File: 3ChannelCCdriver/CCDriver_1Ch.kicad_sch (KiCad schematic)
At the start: 7 parts, among them U1 AL8860WT-7

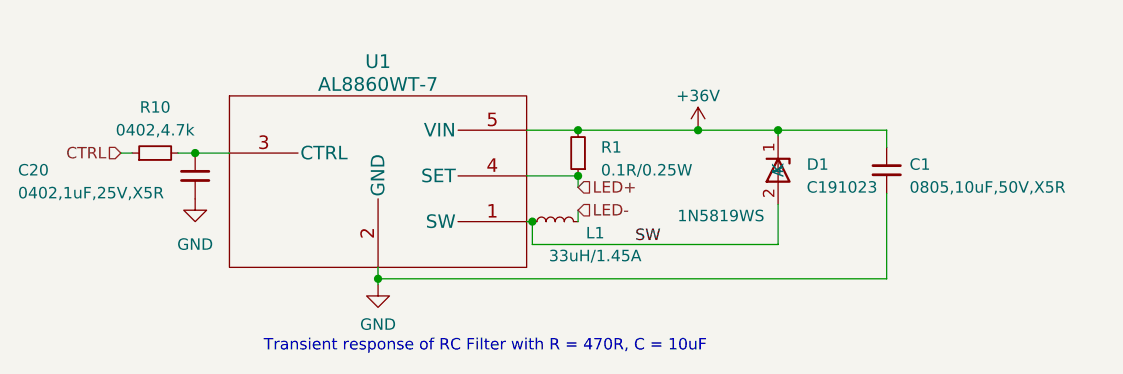
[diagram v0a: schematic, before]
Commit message: neat-ified schematics
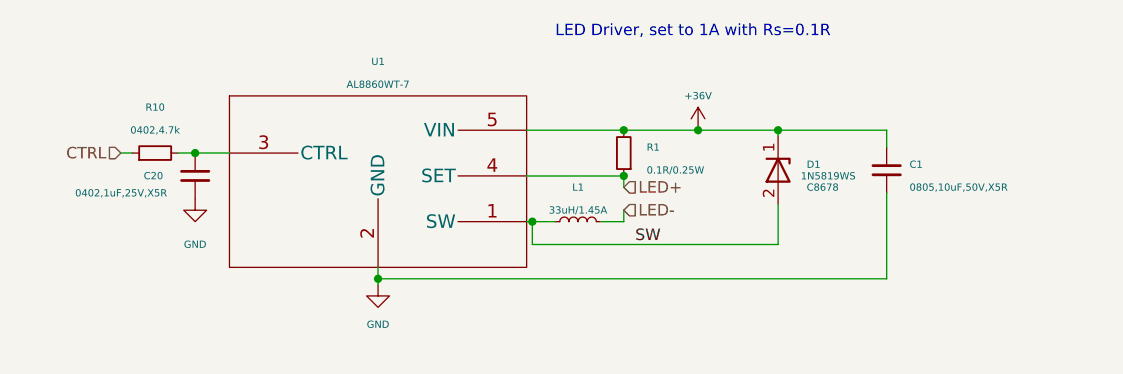
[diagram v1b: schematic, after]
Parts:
- D1: footprint Diode_SMD:D_SOD-323 -> Diode_SMD:D_SMA; LCSC C191023 -> C8678
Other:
- note added: "LED Driver, set to 1A with Rs=0.1R"
- note removed: "Transient response of RC Filter with R = 470R, C = 10uF"
- title: (none) -> 1 Ch CC LED Driver
- moved on the sheet: L1, R1
